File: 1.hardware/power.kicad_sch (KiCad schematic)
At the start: 74 parts, among them IC8 LMR51610XDBVR, J4 12V~48V BAT, J5 12V-48V Jack, SW1 SW_DPST_x2

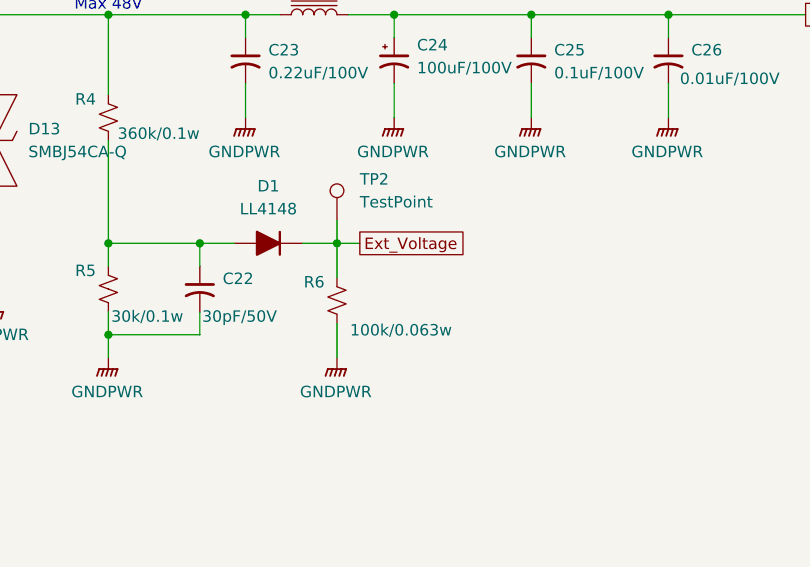
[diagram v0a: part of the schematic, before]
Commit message: 중간 저장
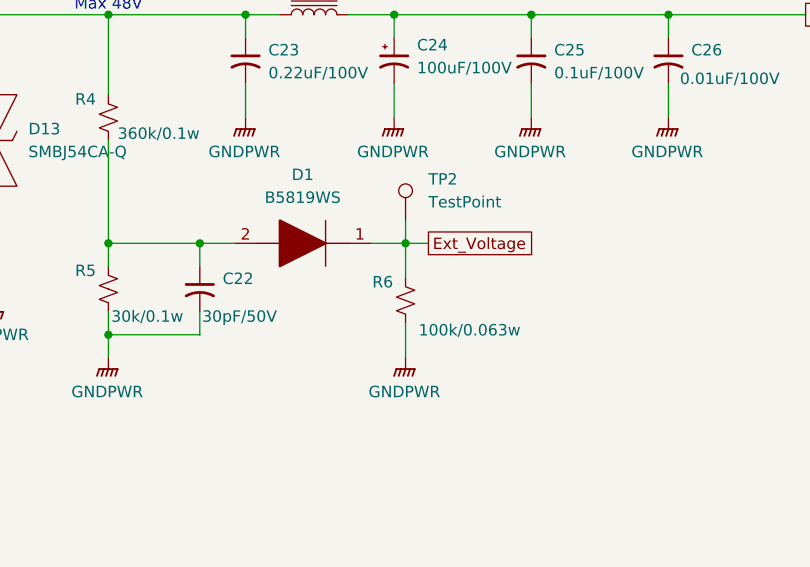
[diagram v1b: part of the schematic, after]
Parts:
- removed D1: LL4148, PCM_Diode_SMD_AKL:D_MiniMELF, symbol PCM_Diode_AKL:LL4148
- added D1: B5819WS, SOD2613X100N, symbol SamacSys_Parts:B5819WS
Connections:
- net Ext_Voltage: now also D1.1
- net at C22.1, R4.1, R5.2: now also D1.2
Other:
- moved on the sheet: R6, TP2
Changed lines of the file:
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@@
 	)
 	(junction
-		(at 116.84 55.88)
+		(at 124.46 55.88)
 		(diameter 0)
 		(color 0 0 0 0)
@@
 	(wire
 		(pts
-			(xy 113.03 55.88) (xy 116.84 55.88)
+			(xy 120.65 55.88) (xy 124.46 55.88)
 		)
 		(stroke
@@
 	(wire
 		(pts
-			(xy 116.84 55.88) (xy 116.84 59.69)
+			(xy 124.46 55.88) (xy 124.46 59.69)
 		)
 		(stroke
@@
 	(wire
 		(pts
-			(xy 116.84 53.34) (xy 116.84 55.88)
+			(xy 124.46 53.34) (xy 124.46 55.88)
 		)
 		(stroke
@@
 	(wire
 		(pts
-			(xy 116.84 64.77) (xy 116.84 68.58)
+			(xy 124.46 64.77) (xy 124.46 68.58)
 		)
 		(stroke
@@
 	(wire
 		(pts
-			(xy 116.84 55.88) (xy 119.38 55.88)
+			(xy 124.46 55.88) (xy 127 55.88)
 		)
 		(stroke
@@
 	(global_label "Ext_Voltage"
 		(shape passive)
-		(at 119.38 55.88 0)
+		(at 127 55.88 0)
 		(fields_autoplaced yes)
 		(effects
@@
 		)
 		(property "Intersheetrefs" "${INTERSHEET_REFS}"
-			(at 132.1394 55.88 0)
+			(at 139.7594 55.88 0)
 			(effects
 				(font
@@
 	)
 	(symbol
+		(lib_id "SamacSys_Parts:B5819WS")
+		(at 120.65 55.88 180)
+		(unit 1)
+		(exclude_from_sim no)
+		(in_bom yes)
+		(on_board yes)
+		(dnp no)
+		(fields_autoplaced yes)
+		(property "Reference" "D1"
+			(at 113.03 48.26 0)
+			(effects
+				(font
+					(size 1.27 1.27)
+				)
+			)
+		)
+		(property "Value" "B5819WS"
+			(at 113.03 50.8 0)
+			(effects
+				(font
+					(size 1.27 1.27)
+				)
+			)
+		)
+		(property "Footprint" "SOD2613X100N"
+			(at 109.22 55.88 0)
+			(effects
+				(font
+					(size 1.27 1.27)
+				)
+				(justify left)
+				(hide yes)
+			)
+		)
+		(property "Datasheet" "https://www.21yangjie.com/ggs/xxh/xxhxtdejg/B5817WS%20THRU%20B5819WS-SOD-323-%E6%B5%B7%E9%B8%A5%E8%84%9A.pdf"
+			(at 109.22 53.34 0)
+			(effects
+				(font
+					(size 1.27 1.27)
+				)
+				(justify left)
+				(hide yes)
+			)
+		)
+		(property "Description" "DIODE SCHOTTKY 40V 1A SOD323"
+			(at 120.65 55.88 0)
+			(effects
+				(font
+					(size 1.27 1.27)
+				)
+				(hide yes)
+			)
+		)
+		(property "Description_1" "DIODE SCHOTTKY 40V 1A SOD323"
+			(at 109.22 50.8 0)
+			(effects
+				(font
+					(size 1.27 1.27)
+				)
+				(justify left)
+				(hide yes)
+			)
+		)
+		(property "Height" "1"
+			(at 109.22 48.26 0)
+			(effects
+				(font
+					(size 1.27 1.27)
+				)
+				(justify left)
+				(hide yes)
+			)
+		)
+		(property "Manufacturer_Name" "Yangzhou Yangjie Electronic Technology Co., Ltd."
+			(at 109.22 45.72 0)
+			(effects
+				(font
+					(size 1.27 1.27)
+				)
+				(justify left)
+				(hide yes)
+			)
+		)
+		(property "Manufacturer_Part_Number" "B5819WS"
+			(at 109.22 43.18 0)
+			(effects
+				(font
+					(size 1.27 1.27)
+				)
+				(justify left)
+				(hide yes)
+			)
+		)
+		(property "Mouser Part Number" ""
+			(at 109.22 40.64 0)
+			(effects
+				(font
+					(size 1.27 1.27)
+				)
+				(justify left)
+				(hide yes)
+			)
+		)
+		(property "Mouser Price/Stock" ""
+			(at 109.22 38.1 0)
+			(effects
+				(font
+					(size 1.27 1.27)
+				)
+				(justify left)
+				(hide yes)
+			)
+		)
+		(property "Arrow Part Number" ""
+			(at 109.22 35.56 0)
+			(effects
+				(font
+					(size 1.27 1.27)
+				)
+				(justify left)
+				(hide yes)
+			)
+		)
+		(property "Arrow Price/Stock" ""
+			(at 109.22 33.02 0)
+			(effects
+				(font
+					(size 1.27 1.27)
+				)
+				(justify left)
+				(hide yes)
+			)
+		)
+		(pin "2"
+		)
+		(pin "1"
+		)
+		(instances
+			(project "bldc_motor_controller"
+				(path "/a25adab6-a8c3-4e0e-8ba9-baac00aaa394/fa552ebf-4859-4df7-97cc-cc5957e0d3a3"
+					(reference "D1")
+					(unit 1)
+				)
+			)
+		)
+	)
+	(symbol
 		(lib_id "power:GNDPWR")
 		(at 78.74 62.23 0)
@@
 	)
 	(symbol
-		(lib_id "PCM_Diode_AKL:LL4148")
-		(at 109.22 55.88 0)
-		(unit 1)
-		(exclude_from_sim no)
-		(in_bom yes)
-		(on_board yes)
-		(dnp no)
-		(fields_autoplaced yes)
-		(property "Reference" "D1"
-			(at 109.22 49.53 0)
-			(effects
-				(font
-					(size 1.27 1.27)
-				)
-			)
-		)
-		(property "Value" "LL4148"
-			(at 109.22 52.07 0)
-			(effects
-				(font
-					(size 1.27 1.27)
-				)
-			)
-		)
-		(property "Footprint" "PCM_Diode_SMD_AKL:D_MiniMELF"
-			(at 109.22 55.88 0)
-			(effects
-				(font
-					(size 1.27 1.27)
-				)
-				(hide yes)
-			)
-		)
-		(property "Datasheet" "https://www.tme.eu/Document/968b88464c4f5d5ff32cd1ca930873a4/LL4148-4448.pdf"
-			(at 109.22 55.88 0)
-			(effects
-				(font
-					(size 1.27 1.27)
-				)
-				(hide yes)
-			)
-		)
-		(property "Description" "MiniMELF Diode, Small Signal, Fast Switching, 75V, 150mA, 4ns, Alternate KiCad Library"
-			(at 109.22 55.88 0)
-			(effects
-				(font
-					(size 1.27 1.27)
-				)
-				(hide yes)
-			)
-		)
-		(pin "1"
-		)
-		(pin "2"
-		)
-		(instances
-			(project ""
-				(path "/a25adab6-a8c3-4e0e-8ba9-baac00aaa394/fa552ebf-4859-4df7-97cc-cc5957e0d3a3"
-					(reference "D1")
-					(unit 1)
-				)
-			)
-		)
-	)
-	(symbol
 		(lib_id "Device:L_Iron")
 		(at 162.56 127 90)
@@
 	(symbol
 		(lib_id "Device:R_Small_US")
-		(at 116.84 62.23 180)
+		(at 124.46 62.23 180)
 		(unit 1)
 		(exclude_from_sim no)
@@
 		(dnp no)
 		(property "Reference" "R6"
-			(at 114.3 60.198 0)
+			(at 121.92 60.198 0)
 			(effects
 				(font
@@
 		)
 		(property "Value" "100k/0.063w"
-			(at 123.952 65.532 0)
+			(at 131.572 65.532 0)
 			(effects
 				(font
@@
 		)
 		(property "Footprint" ""
-			(at 116.84 62.23 0)
+			(at 124.46 62.23 0)
 			(effects
 				(font
@@
 		)
 		(property "Datasheet" "~"
-			(at 116.84 62.23 0)
+			(at 124.46 62.23 0)
 			(effects
 				(font
@@
 		)
 		(property "Description" "Resistor, small US symbol"
-			(at 116.84 62.23 0)
+			(at 124.46 62.23 0)
 			(effects
 				(font
@@
 	(symbol
 		(lib_id "Connector:TestPoint")
-		(at 116.84 53.34 0)
+		(at 124.46 53.34 0)
 		(unit 1)
 		(exclude_from_sim no)
@@
 		(fields_autoplaced yes)
 		(property "Reference" "TP2"
-			(at 119.38 48.7679 0)
+			(at 127 48.7679 0)
 			(effects
 				(font
@@
 		)
 		(property "Value" "TestPoint"
-			(at 119.38 51.3079 0)
+			(at 127 51.3079 0)
 			(effects
 				(font
@@
 		)
 		(property "Footprint" ""
-			(at 121.92 53.34 0)
+			(at 129.54 53.34 0)
 			(effects
 				(font
@@
 		)
 		(property "Datasheet" "~"
-			(at 121.92 53.34 0)
+			(at 129.54 53.34 0)
 			(effects
 				(font
@@
 		)
 		(property "Description" "test point"
-			(at 116.84 53.34 0)
+			(at 124.46 53.34 0)
 			(effects
 				(font
@@
 	(symbol
 		(lib_id "power:GNDPWR")
-		(at 116.84 68.58 0)
+		(at 124.46 68.58 0)
 		(unit 1)
 		(exclude_from_sim no)
@@
 		(fields_autoplaced yes)
 		(property "Reference" "#PWR024"
-			(at 116.84 73.66 0)
+			(at 124.46 73.66 0)
 			(effects
 				(font
@@
 		)
 		(property "Value" "GNDPWR"
-			(at 116.713 72.39 0)
+			(at 124.333 72.39 0)
 			(effects
 				(font
@@
 		)
 		(property "Footprint" ""
-			(at 116.84 69.85 0)
+			(at 124.46 69.85 0)
 			(effects
 				(font
@@
 		)
 		(property "Datasheet" ""
-			(at 116.84 69.85 0)
+			(at 124.46 69.85 0)
 			(effects
 				(font
@@
 		)
 		(property "Description" "Power symbol creates a global label with name \"GNDPWR\" , global ground"
-			(at 116.84 68.58 0)
+			(at 124.46 68.58 0)
 			(effects
 				(font
